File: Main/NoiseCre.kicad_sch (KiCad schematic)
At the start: 57 parts, among them J1 Out, J2 CV In, J3 Conn_01x06, J4 Conn_01x06, J5 In, Q1 BC548, Q2 2N3906, Q3 2N3906, SW1 SW_DPDT_x2, U1 TL072, U2 LM13700

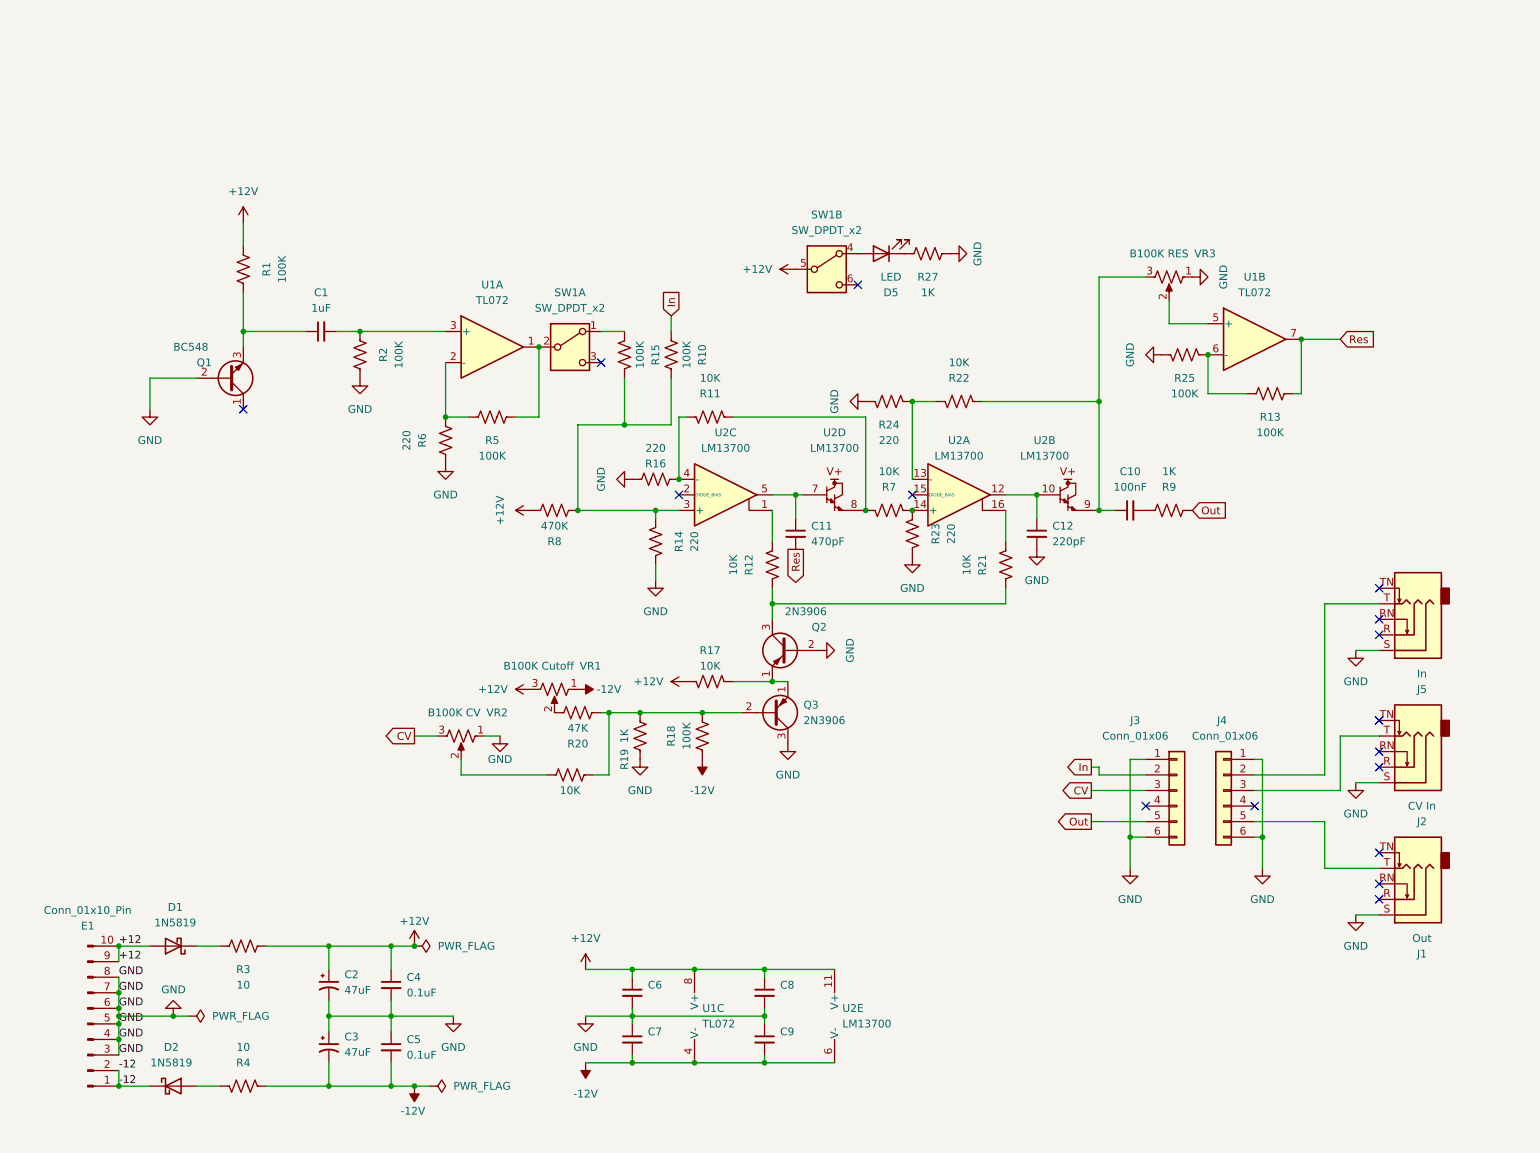
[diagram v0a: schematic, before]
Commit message: Upload Schematics
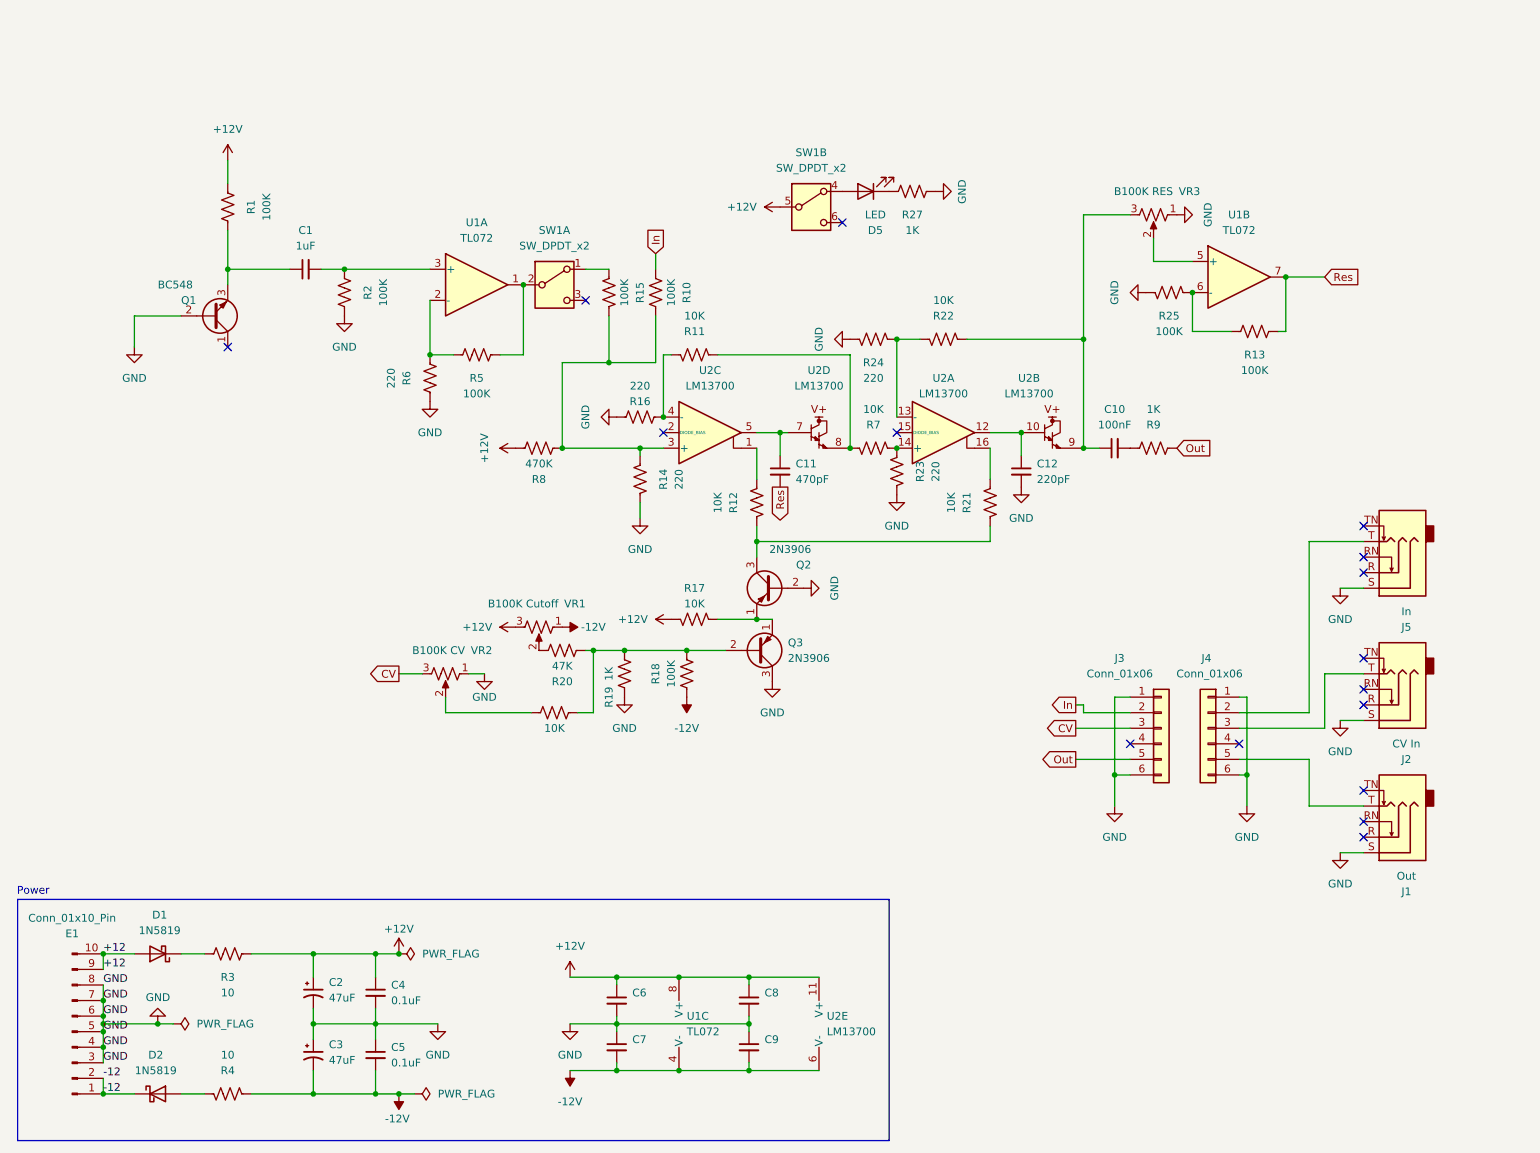
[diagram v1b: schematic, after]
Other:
- note added: "Power"
- moved on the sheet: C1, C10, C11, C12, C2, C3, C4, C5, C6, C7, C8, C9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

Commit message: Updated gain output
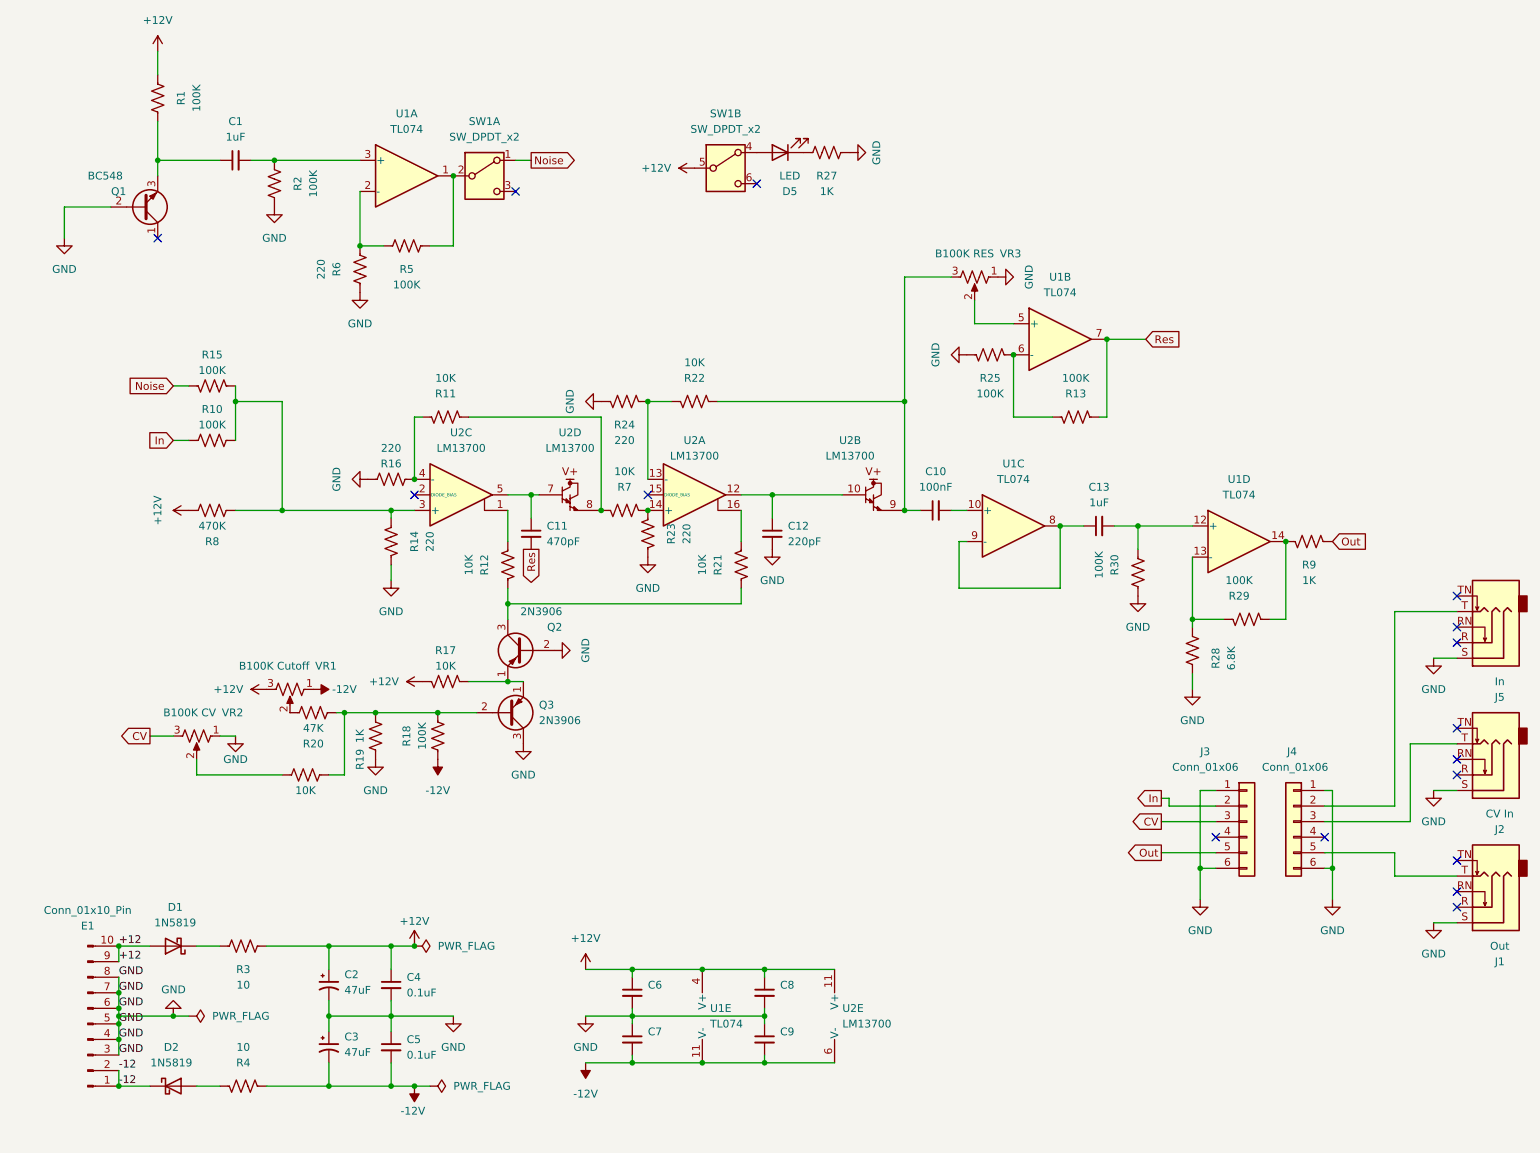
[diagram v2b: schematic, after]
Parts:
- removed U1: TL072, AO_tht:DIP-8_W7.62mm_Socket_LongPads, symbol Amplifier_Operational:TL072
- added C13: 1uF, Capacitor_THT:C_Rect_L7.2mm_W5.5mm_P5.00mm_FKS2_FKP2_MKS2_MKP2, symbol Device:C_Small
- added R28: 6.8K, AO_tht:R_Axial_DIN0207_L6.3mm_D2.5mm_P10.16mm_Horizontal, symbol Device:R_US
- added R29, R30: 100K, AO_tht:R_Axial_DIN0207_L6.3mm_D2.5mm_P10.16mm_Horizontal, symbol Device:R_US
- added U1: TL074, AO_tht:DIP-14_W7.62mm_Socket_LongPads, symbol Amplifier_Operational:TL074
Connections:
- net +12V: now also U1.4 (V+)
- net -12V: now also U1.11 (V-)
- net GND: now also R28.1, R30.2
- net Res: now also U1.7
- net at C1.2, R2.2: now also U1.3 (+)
- net at R13.1, R25.1: now also U1.6 (-)
- net Noise: now reaches R15.2, SW1.1 (A)
- net at R5.2, SW1.2 (B): now also U1.1
- net at R5.1, R6.1: now also U1.2 (-)
- net at VR3.2: now also U1.5 (+)
- net at R9.2: now also R29.2, U1.14; no longer C10.2
- new net: C13.1, U1.8, U1.9 (-)
- new net: C13.2, R30.1, U1.12 (+)
- new net: R28.2, R29.1, U1.13 (-)
- new net: C10.2, U1.10 (+)
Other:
- note removed: "Power"
- moved on the sheet: C1, C10, C11, C12, C2, C3, C4, C5, C6, C7, C8, C9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
